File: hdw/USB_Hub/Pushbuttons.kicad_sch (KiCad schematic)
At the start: 10 parts

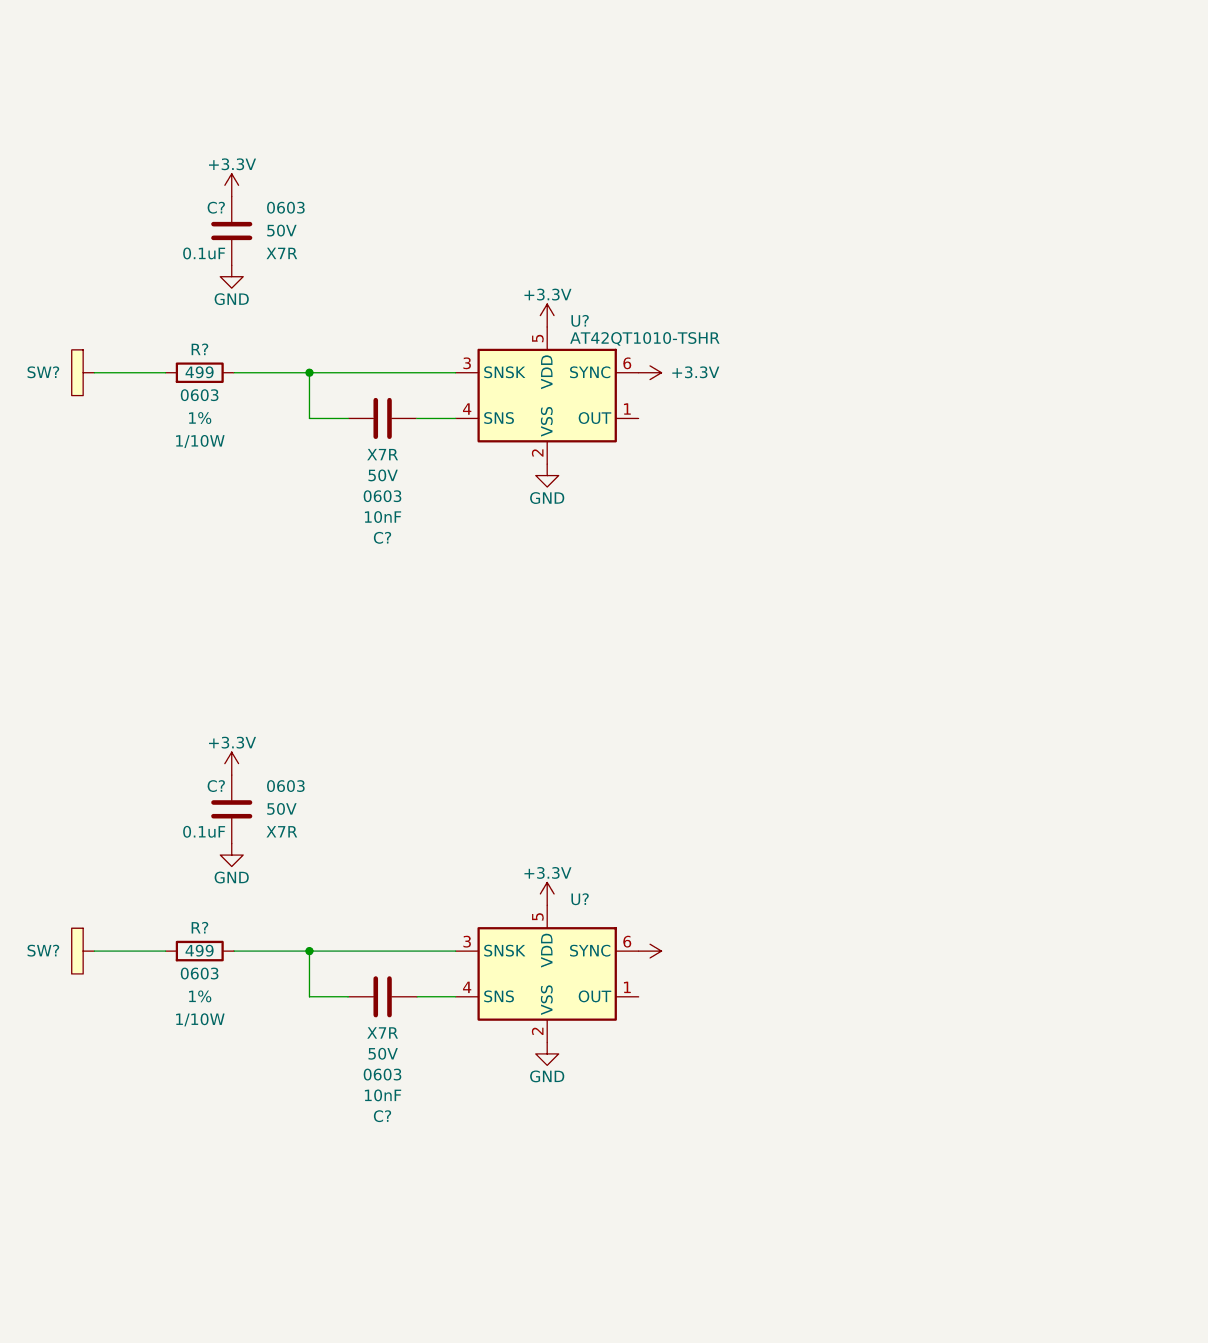
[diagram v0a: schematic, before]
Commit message: much more schematic progress
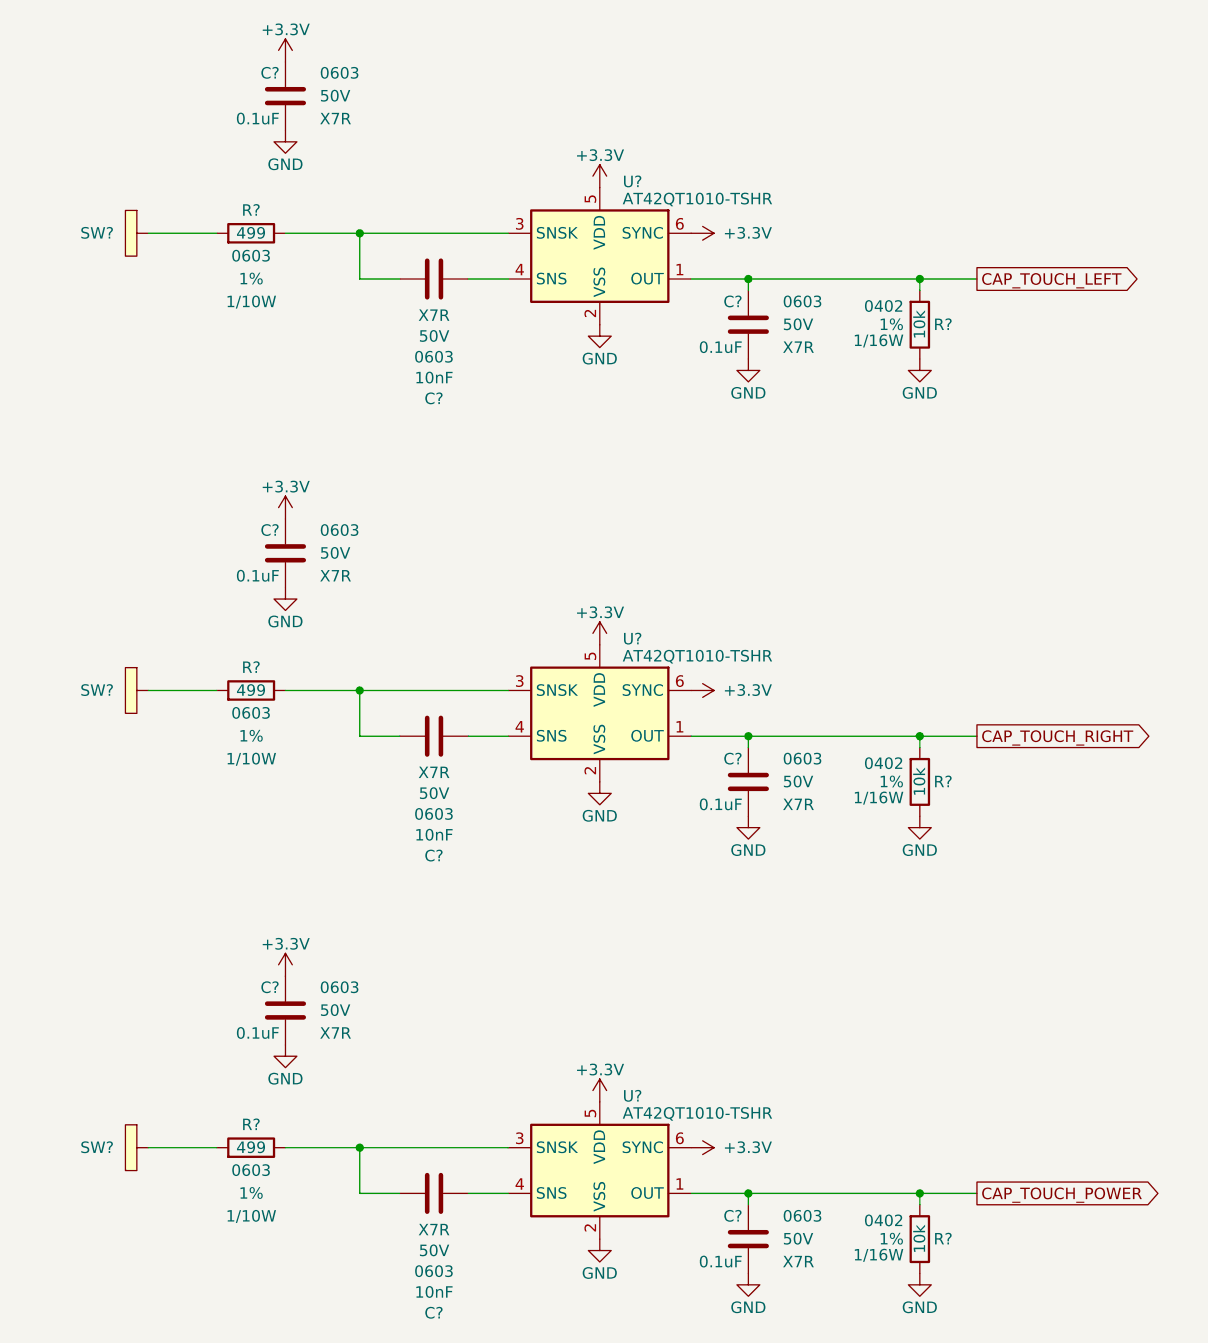
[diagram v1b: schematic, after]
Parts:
- removed C?: 10nF, Capacitors_SMD:C_0603, symbol Custom_Library:C_Custom
- removed C?: 0.1uF, Capacitors_SMD:C_0603, symbol Custom_Library:C_Custom
- removed R?: 499, Resistors_SMD:R_0603, symbol Custom_Library:R_Custom
- removed SW?: Cap_Touch, Custom Footprints Library:Capacitive_Touch_Pad, symbol Custom_Library:Cap_Touch
- removed U?: AT42QT1010-TSHR, TO_SOT_Packages_SMD:SOT-23-6, symbol Sensor_Touch:AT42QT1010-TSHR
- added C? (x2): 10nF, Capacitors_SMD:C_0603, symbol Custom_Library:C_Custom
- added C? (x5): 0.1uF, Capacitors_SMD:C_0603, symbol Custom_Library:C_Custom
- added R? (x3): 10k, Resistors_SMD:R_0402, symbol Custom_Library:R_Custom
- added R? (x2): 499, Resistors_SMD:R_0603, symbol Custom_Library:R_Custom
- added SW? (x2): Cap_Touch, Custom Footprints Library:Capacitive_Touch_Pad, symbol Custom_Library:Cap_Touch
- added U? (x2): AT42QT1010-TSHR, TO_SOT_Packages_SMD:SOT-23-6, symbol Sensor_Touch:AT42QT1010-TSHR
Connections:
- net +3.3V: now also C?.1, C?.1, U?.5 (VDD), U?.5 (VDD), U?.6 (SYNC), U?.6 (SYNC)
- net GND: now also C?.2, C?.2, C?.2, C?.2, C?.2, R?.2, R?.2, R?.2, U?.2 (VSS), U?.2 (VSS)
- net CAP_TOUCH_LEFT: now reaches U?.1 (OUT)
- net CAP_TOUCH_LEFT: now also C?.1, R?.1
- new net: C?.1, U?.4 (SNS) (x2)
- new net: C?.2, R?.2, U?.3 (SNSK) (x2)
- new net: R?.1, SW?.1 (TP) (x2)
- new net CAP_TOUCH_POWER: C?.1, R?.1, U?.1 (OUT)
- new net CAP_TOUCH_RIGHT: C?.1, R?.1, U?.1 (OUT)
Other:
- moved on the sheet: C?, R?, SW?, U?
